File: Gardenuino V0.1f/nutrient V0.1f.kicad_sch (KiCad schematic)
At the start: 86 parts, among them J1 Conn_01x04_Male, J10 Conn_01x01_Male, J2 Conn_01x04_Male, J3 Conn_01x04_Female, J4 Conn_01x04_Male, J5 Conn_01x04_Female, J6 Conn_01x04_Female, J7 Conn_01x03_Male, J8 Conn_01x03_Male, J9 Conn_01x01_Male, P1 SolderJumper_2_Bridged, P2 SolderJumper_2_Bridged, P3 SolderJumper_2_Bridged, P4 SolderJumper_2_Bridged, Q1 Q_NMOS_DGS, Q10 Q_NMOS_DGS, Q2 Q_NMOS_DGS, Q3 Q_NMOS_DGS, Q4 Q_NMOS_DGS, Q5 Q_NMOS_DGS, Q6 Q_NMOS_DGS, Q7 Q_NMOS_DGS, Q8 2N3904, U1 23LC512, U2 DS1307+, Y1 Crystal_Small

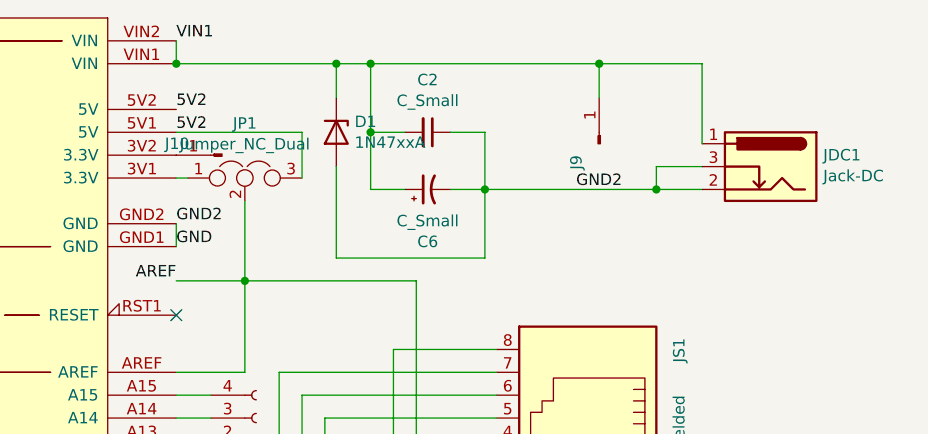
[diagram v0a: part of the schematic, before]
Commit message: SpectDrone Development
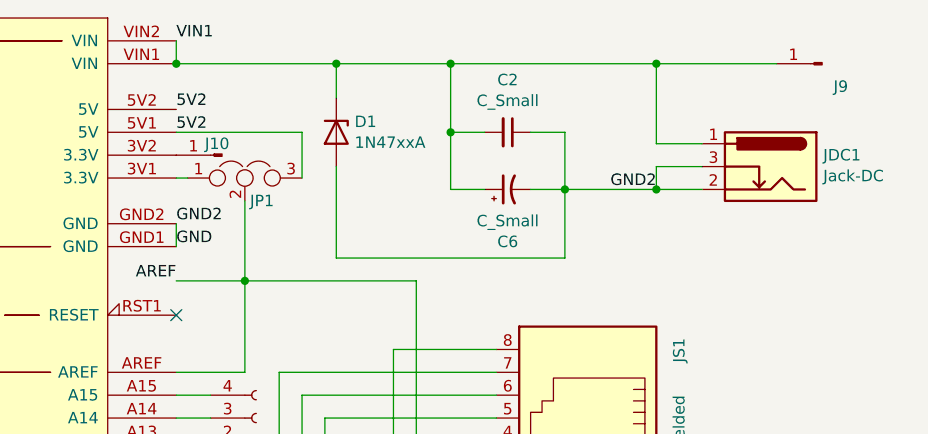
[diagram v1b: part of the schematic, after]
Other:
- moved on the sheet: C2, C6, J9
